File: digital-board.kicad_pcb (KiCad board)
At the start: 2 copper layers, 200 x 150 mm, 238 parts, among them IC1 ATMEGA6450-A, J1 CONN_20X2, Q1 2N3904, Q2 2N3904, SW15 TACT_SWITCH, SW16 TACT_SWITCH, SW17 TACT_SWITCH, SW18 TACT_SWITCH, SW19 TACT_SWITCH, SW20 TACT_SWITCH, SW21 TACT_SWITCH, SW22 TACT_SWITCH, SW23 TACT_SWITCH, U1 DG419, U10 74LVC1G32, U12 74AC595, U13 74AC595, U14 74HC165, U15 74AC595, U16 74AC595, U2 74HC4067, U3 R-78E5.0-1.0, U4 74HC4067, U5 74LS573, U6 74LS573, U7 74LVC2G04, U8 74AC595, U9 74HC165, X1 MIDI OUT, X2 MIDI IN, X3 MIDI THRU

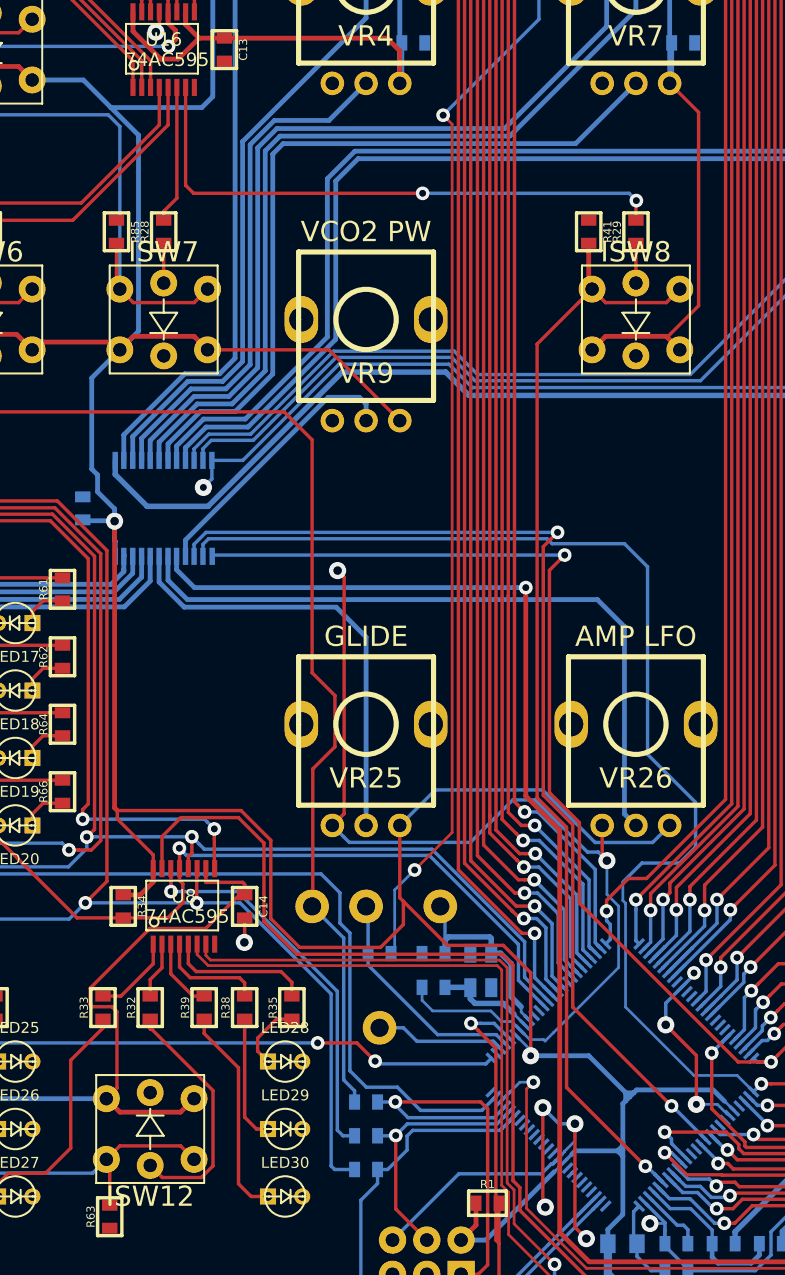
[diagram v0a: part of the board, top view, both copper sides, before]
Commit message: last save before silk screen edit in 5112
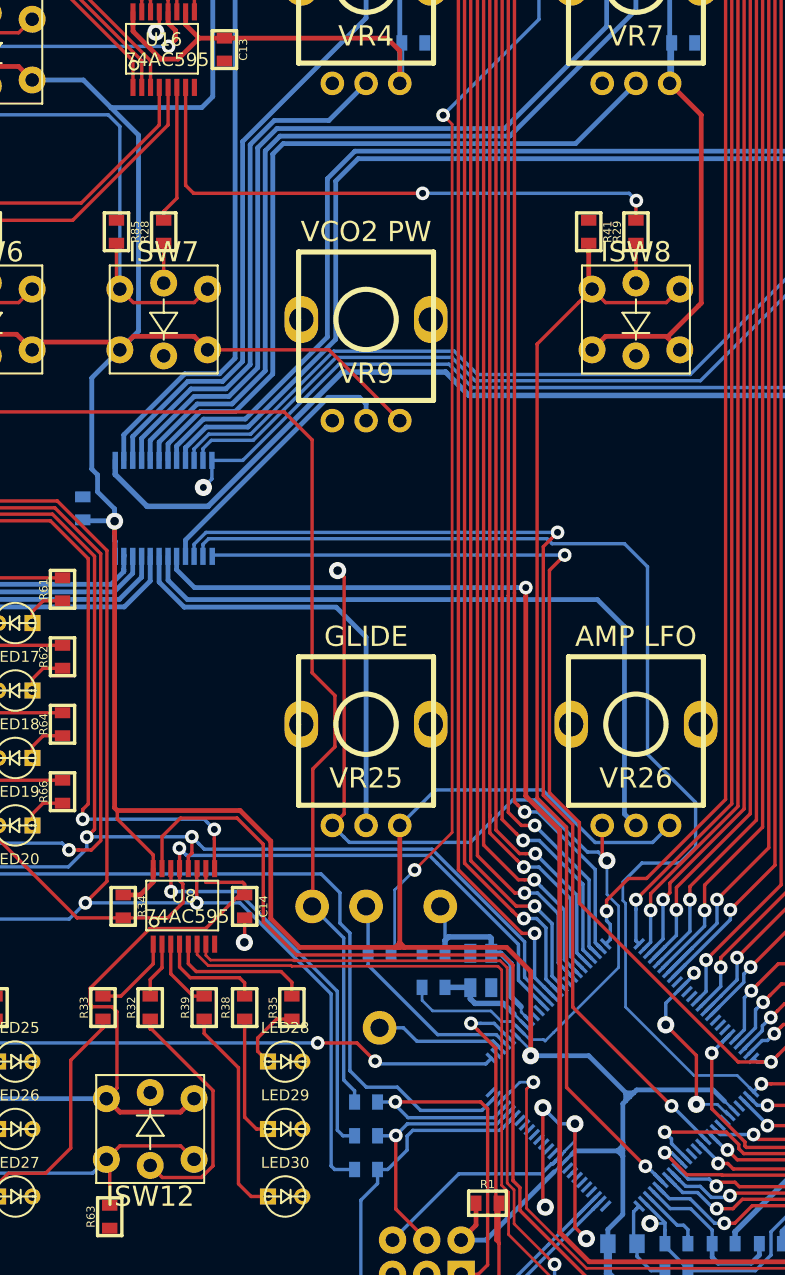
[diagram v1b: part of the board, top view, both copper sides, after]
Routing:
- net +5V: track 1830.1 -> 1830.7 mm
